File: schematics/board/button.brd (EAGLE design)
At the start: 4.5 x 10 mm, 1 part

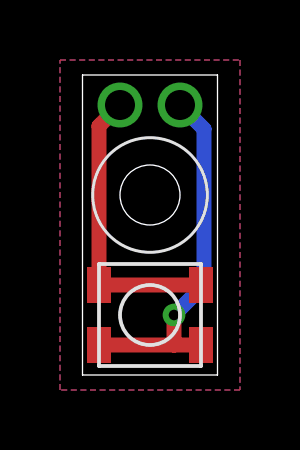
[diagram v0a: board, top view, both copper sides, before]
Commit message: Еще раз проверил все платы и подготовил для производства в Резоните
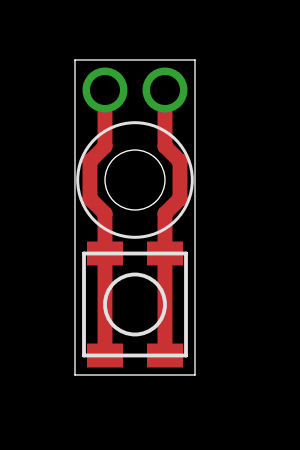
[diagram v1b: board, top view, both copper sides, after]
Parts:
- moved U$1 0.61 mm to (2.00, 2.35), turned to 90 degrees
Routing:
- net P2: track 12.1 -> 9.26 mm, vias 2 -> 1
- removed copper zone on layer 1, net P1
- removed copper zone on layer 16, net P2
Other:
- board size 4.5 x 10 mm -> 4 x 10.5 mm
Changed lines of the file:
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@@
 <board>
 <plain>
-<wire x1="0.25" y1="0" x2="4.75" y2="0" width="0" layer="20"/>
-<wire x1="4.75" y1="0" x2="4.75" y2="10" width="0" layer="20"/>
-<wire x1="4.75" y1="10" x2="0.25" y2="10" width="0" layer="20"/>
-<wire x1="0.25" y1="10" x2="0.25" y2="0" width="0" layer="20"/>
-<hole x="2.5" y="6" drill="2"/>
-<circle x="2.5" y="6" radius="1.910496875" width="0.1" layer="21"/>
+<wire x1="0" y1="0" x2="4" y2="0" width="0" layer="20"/>
+<wire x1="4" y1="0" x2="4" y2="10.5" width="0" layer="20"/>
+<wire x1="4" y1="10.5" x2="0" y2="10.5" width="0" layer="20"/>
+<wire x1="0" y1="10.5" x2="0" y2="0" width="0" layer="20"/>
+<hole x="2" y="6.5" drill="2"/>
+<circle x="2" y="6.5" radius="1.910496875" width="0.1" layer="21"/>
 </plain>
 <attributes>
@@
 <param name="mdViaViaSameLayer" value="6mil"/>
 <param name="mnLayersViaInSmd" value="2"/>
-<param name="mdCopperDimension" value="0.1mm"/>
+<param name="mdCopperDimension" value="0.25mm"/>
 <param name="mdDrill" value="6mil"/>
 <param name="mdSmdStop" value="0mil"/>
@@
 </autorouter>
 <elements>
-<element name="U$1" library="NEON-BLADE-2023" package="BTN-VS-CUT" value="BTN_VERY_SMALLCUT" x="2.5" y="2" smashed="yes"/>
+<element name="U$1" library="NEON-BLADE-2023" package="BTN-VS-CUT" value="BTN_VERY_SMALLCUT" x="2" y="2.35" smashed="yes" rot="R90"/>
 </elements>
 <signals>
@@
 <contactref element="U$1" pad="P$1"/>
 <contactref element="U$1" pad="P$2"/>
-<via x="1.5" y="9" extent="1-16" drill="1"/>
-<wire x1="4.2" y1="3" x2="0.8" y2="3" width="0.5" layer="1"/>
-<wire x1="1.5" y1="9" x2="0.8" y2="8.3" width="0.5" layer="1"/>
-<wire x1="0.8" y1="8.3" x2="0.8" y2="3" width="0.5" layer="1"/>
-<polygon width="0.2" layer="1">
-<vertex x="-0.5" y="10.5"/>
-<vertex x="5.5" y="10.5"/>
-<vertex x="5.5" y="-0.5"/>
-<vertex x="-0.5" y="-0.5"/>
-</polygon>
+<via x="1" y="9.5" extent="1-16" drill="1"/>
+<wire x1="1" y1="4.05" x2="1" y2="5.378675" width="0.5" layer="1"/>
+<wire x1="1" y1="5.378675" x2="0.5" y2="5.878675" width="0.5" layer="1"/>
+<wire x1="0.5" y1="5.878675" x2="0.5" y2="7.121325" width="0.5" layer="1"/>
+<wire x1="0.5" y1="7.121325" x2="1" y2="7.621325" width="0.5" layer="1"/>
+<wire x1="1" y1="7.621325" x2="1" y2="9.5" width="0.5" layer="1"/>
+<wire x1="1" y1="0.65" x2="1" y2="4.05" width="0.5" layer="1"/>
 </signal>
 <signal name="P2">
 <contactref element="U$1" pad="P$3"/>
 <contactref element="U$1" pad="P$4"/>
-<via x="3.5" y="9" extent="1-16" drill="1"/>
-<wire x1="4.2" y1="1" x2="3.3" y2="1" width="0.5" layer="1"/>
-<wire x1="3.3" y1="1" x2="0.8" y2="1" width="0.5" layer="1"/>
-<wire x1="3.3" y1="1" x2="3.3" y2="2" width="0.5" layer="1"/>
-<via x="3.3" y="2" extent="1-16" drill="0.35"/>
-<wire x1="3.3" y1="2" x2="4.3" y2="3" width="0.5" layer="16"/>
-<wire x1="4.3" y1="8.2" x2="3.5" y2="9" width="0.5" layer="16"/>
-<wire x1="4.3" y1="3" x2="4.3" y2="8.2" width="0.5" layer="16"/>
-<polygon width="0.2" layer="16">
-<vertex x="-0.5" y="10.5"/>
-<vertex x="5.5" y="10.5"/>
-<vertex x="5.5" y="-0.5"/>
-<vertex x="-0.5" y="-0.5"/>
-</polygon>
+<via x="3" y="9.5" extent="1-16" drill="1"/>
+<wire x1="3" y1="9.5" x2="3" y2="7.621325" width="0.5" layer="1"/>
+<wire x1="3" y1="7.621325" x2="3.5" y2="7.121325" width="0.5" layer="1"/>
+<wire x1="3.5" y1="7.121325" x2="3.5" y2="5.878675" width="0.5" layer="1"/>
+<wire x1="3.5" y1="5.878675" x2="3" y2="5.378675" width="0.5" layer="1"/>
+<wire x1="3" y1="5.378675" x2="3" y2="4.05" width="0.5" layer="1"/>
+<wire x1="3" y1="0.65" x2="3" y2="4.05" width="0.5" layer="1"/>
 </signal>
 </signals>
